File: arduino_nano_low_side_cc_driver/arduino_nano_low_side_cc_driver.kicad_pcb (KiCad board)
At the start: 2 copper layers, 83.5 x 48.6 mm, 37 parts, among them J1 Conn_01x06_Pin, J2 Conn_01x02_Pin, J3 Barrel_Jack, J4 Conn_01x02_Pin, Q1 IRF540N, Q2 IRF540N, U1 L7805, U2 PC817, U3 LM358, U4 PC817

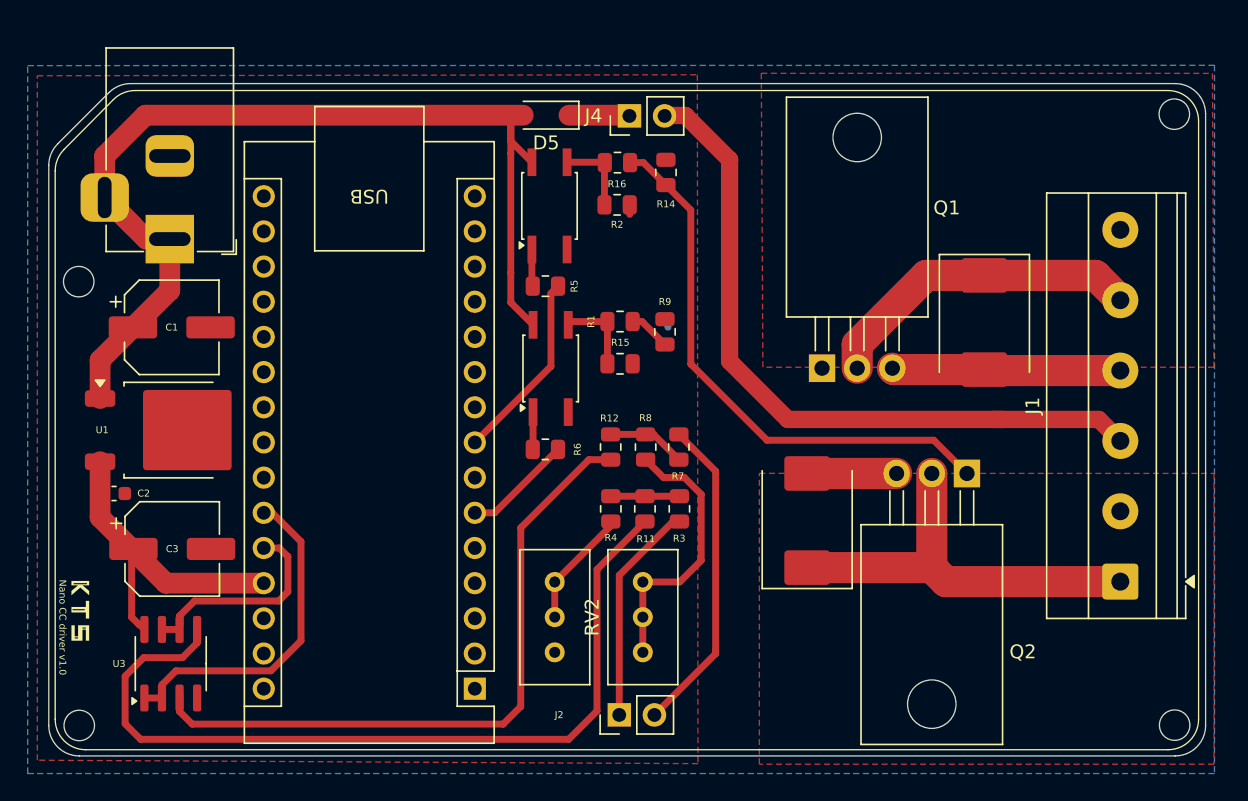
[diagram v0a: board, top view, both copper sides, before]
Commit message: v1.0.0
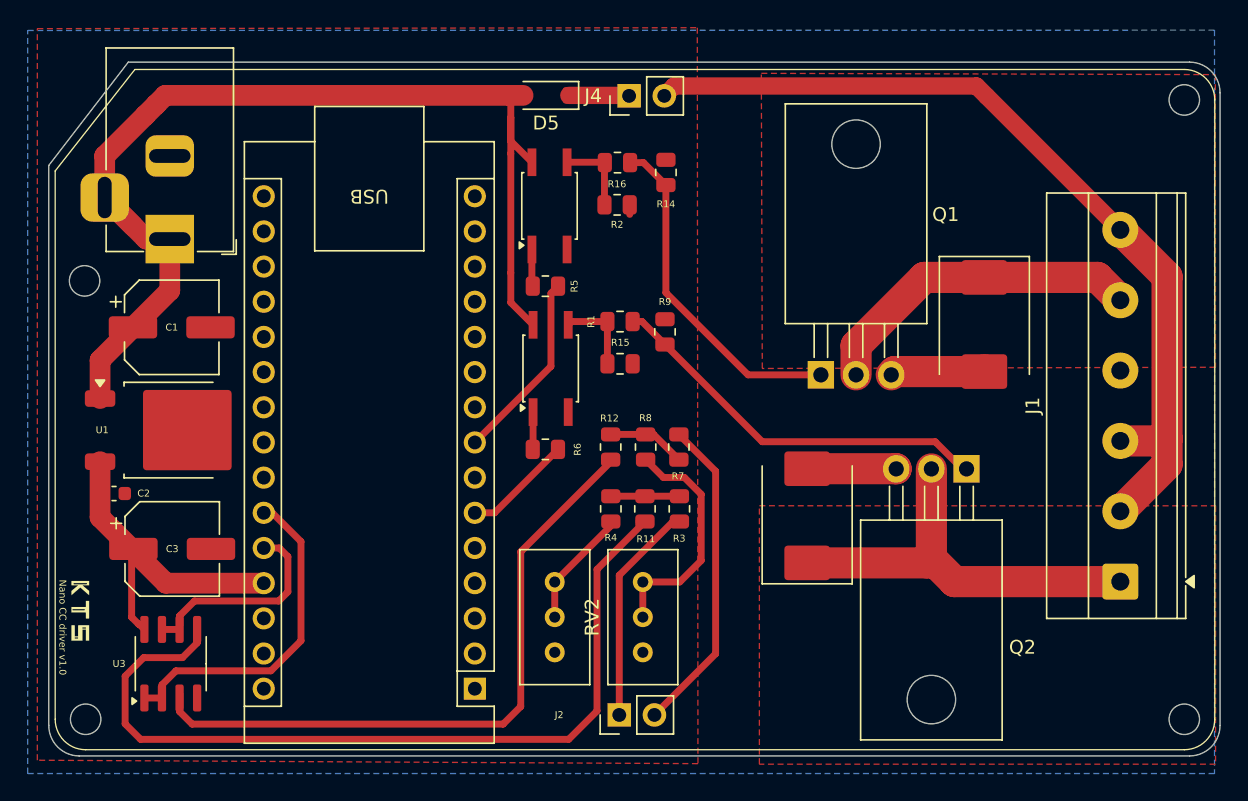
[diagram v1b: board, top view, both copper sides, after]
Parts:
- moved J4 1.45 mm to (170.9, 81.5)
- moved D5 1.43 mm to (164.9, 81.5)
- moved REF** 1.25 mm to (211.0, 81.8)
- moved REF** 0.81 mm to (211.0, 126.5)
- moved REF** 0.64 mm to (131.7, 126.5)
- moved Q1 0.49 mm to (184.8, 101.7)
- moved REF** 0.43 mm to (131.6, 94.9)
- moved D2 0.34 mm to (183.8, 111.9)
- moved Q2 0.33 mm to (195.3, 108.5)
- moved D1 0.14 mm to (196.6, 98.0)
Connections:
- D1 pad 1: L1b -> L2b
- D2 pad 1: L2b -> L1b
- J1 pad 1: L2b -> L1b
- J1 pad 5: L1b -> L2b
- J3 pad 3: (no net) -> 12V
- Q1 pad 2: L1b -> L2b
- Q2 pad 2: L2b -> L1b
- R1 pad 2: Net-(Q1-G) -> Net-(Q2-G)
- R14 pad 2: Net-(Q2-G) -> Net-(Q1-G)
- R16 pad 2: Net-(Q2-G) -> Net-(Q1-G)
- R9 pad 2: Net-(Q1-G) -> Net-(Q2-G)
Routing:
- net Net-(Q1-G): track 3.17 -> 24.8 mm
- net L1a: track 51.7 -> 64.1 mm
- net Net-(Q2-G): track 40.1 -> 28.7 mm
- net GND: track 23.0 -> 13.5 mm
- net L1b: track 23.5 -> 29.9 mm
- net L2b: track 29.8 -> 23.9 mm
- net Net-(R8-Pad1): track 19.8 -> 17.2 mm
- net 12V: track 77.2 -> 79.4 mm
- net Net-(U3A-+): track 49.5 -> 48.6 mm
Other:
- board size 83.5 x 48.6 mm -> 84.6 x 50.1 mm
